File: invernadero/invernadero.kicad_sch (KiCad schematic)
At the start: 25 parts, among them J1 Conn_02x20_Odd_Even, J10 Conn_01x02_Socket, J2 Conn_02x20_Odd_Even, J3 Conn_01x08_Pin, J4 Conn_01x16_Socket, J5 Conn_01x04_Socket, J6 Conn_01x02_Socket, J7 Conn_01x02_Socket, J8 Conn_01x03_Socket, J9 Conn_01x02_Socket, Q1 NPN

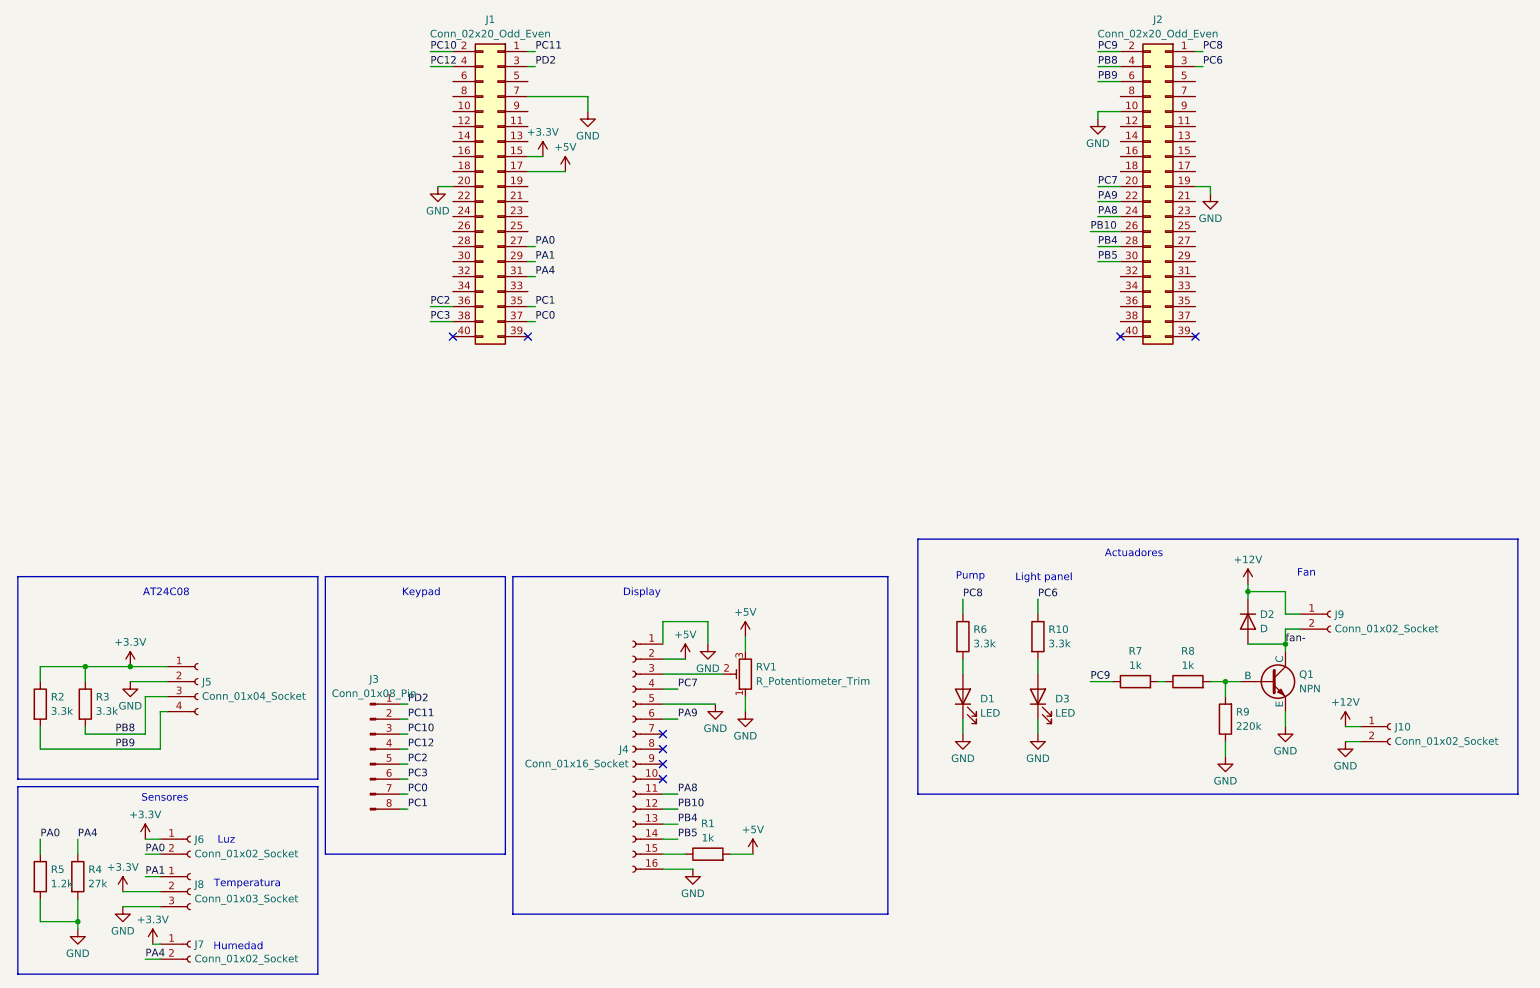
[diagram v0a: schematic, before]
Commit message: PCB actualizado
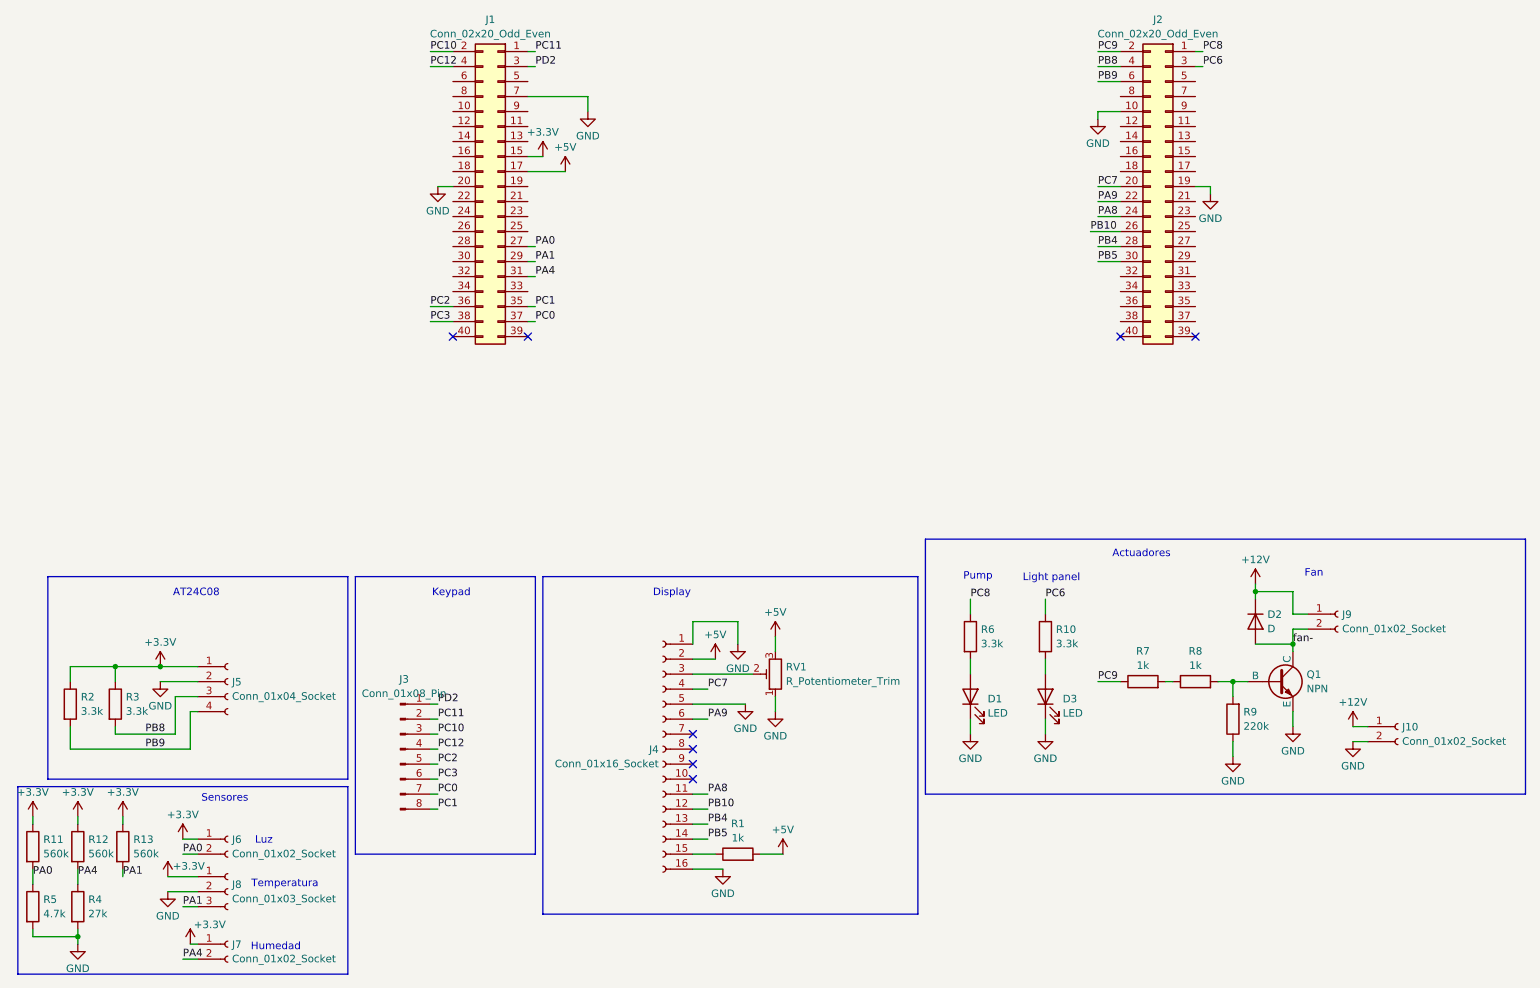
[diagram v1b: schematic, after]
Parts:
- added R11, R12, R13: 560k, Resistor_THT:R_Axial_DIN0207_L6.3mm_D2.5mm_P7.62mm_Horizontal, symbol Device:R
- R5: value 1.2k -> 4.7k
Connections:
- net +3.3V: now also J8.1 (Pin_1), R11.1, R12.1, R13.1; no longer J8.2 (Pin_2)
- net GND: now also J8.2 (Pin_2); no longer J8.3 (Pin_3)
- net PA0: now also R11.2
- net PA1: now also J8.3 (Pin_3), R13.2; no longer J8.1 (Pin_1)
- net PA4: now also R12.2
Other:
- moved on the sheet: D1, D2, D3, J10, J3, J4, J5, J6, J7, J8, J9, Q1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
